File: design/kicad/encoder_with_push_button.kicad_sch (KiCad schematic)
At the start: 1 part

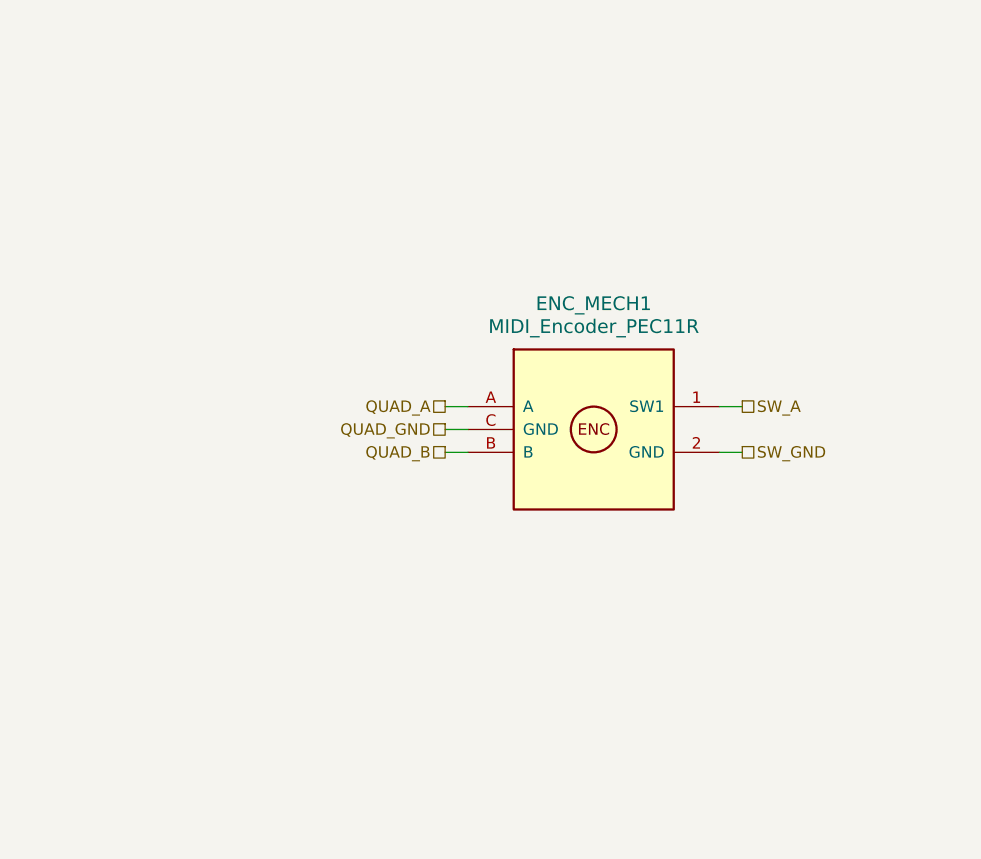
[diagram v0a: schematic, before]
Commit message: Refactor code structure for improved readability and maintainability
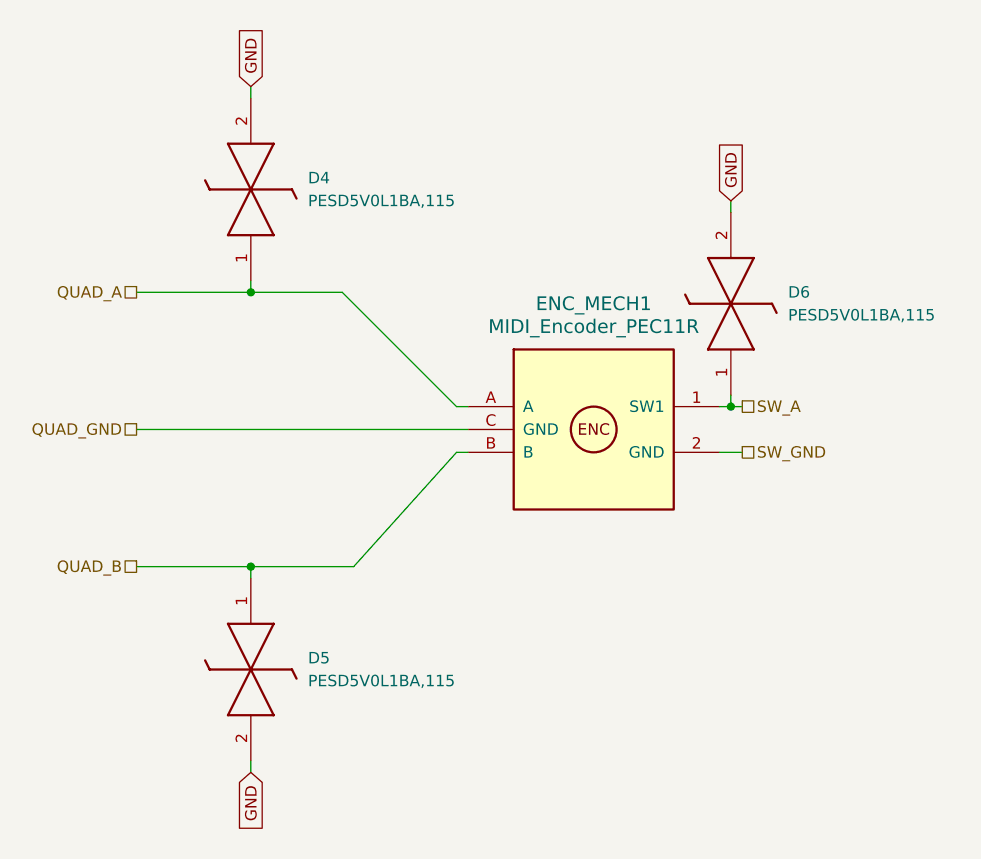
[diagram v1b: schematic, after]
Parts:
- added D4, D5, D6: PESD5V0L1BA,115, KiCad:SOD2512X110N, symbol PESD5V0L1BA_115:PESD5V0L1BA,115
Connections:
- net QUAD_A: now also D4.1 (K1)
- net QUAD_B: now also D5.1 (K1)
- net SW_A: now also D6.1 (K1)
- new net GND: D4.2 (K2), D5.2 (K2), D6.2 (K2)
